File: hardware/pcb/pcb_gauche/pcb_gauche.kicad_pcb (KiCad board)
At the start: 2 copper layers, 28 x 56 mm, 14 parts, among them P1 TE-FFC-10-0.5

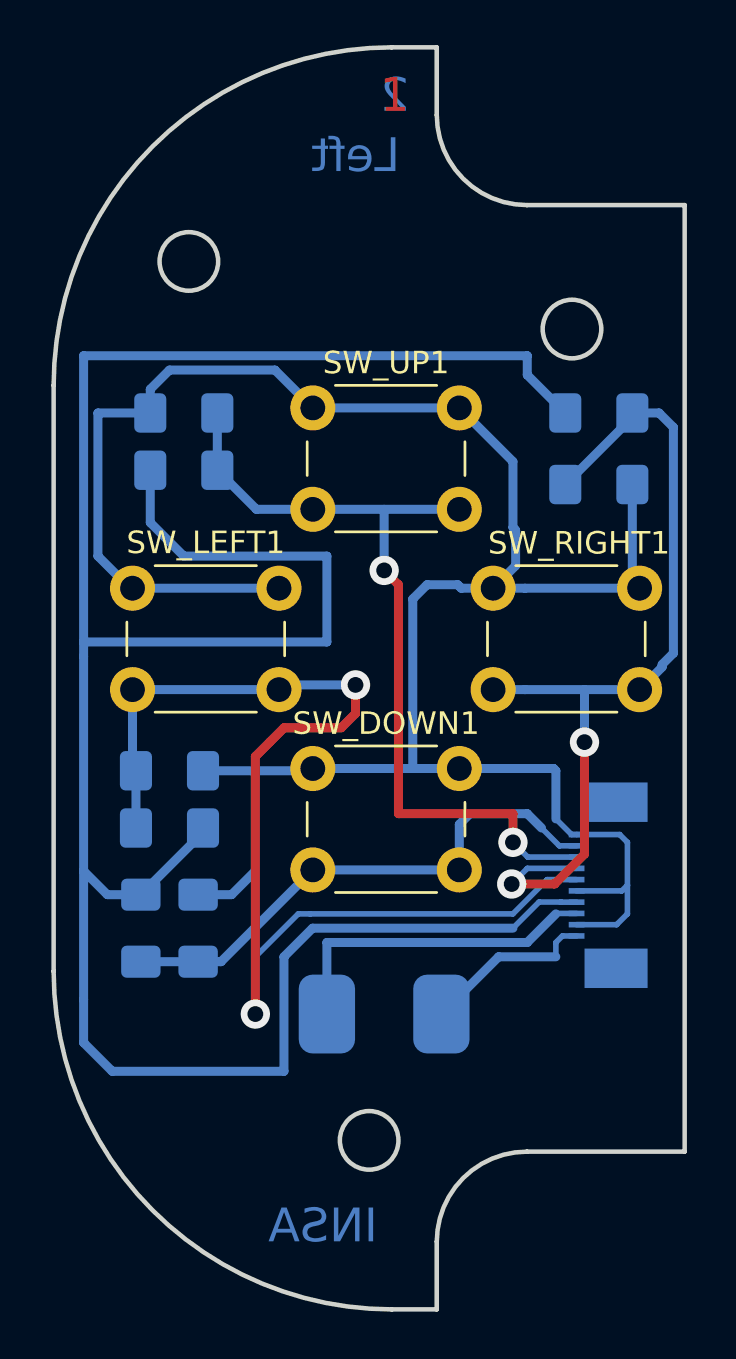
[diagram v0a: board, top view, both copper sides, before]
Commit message: mise a jour des pcb et design mecaniques
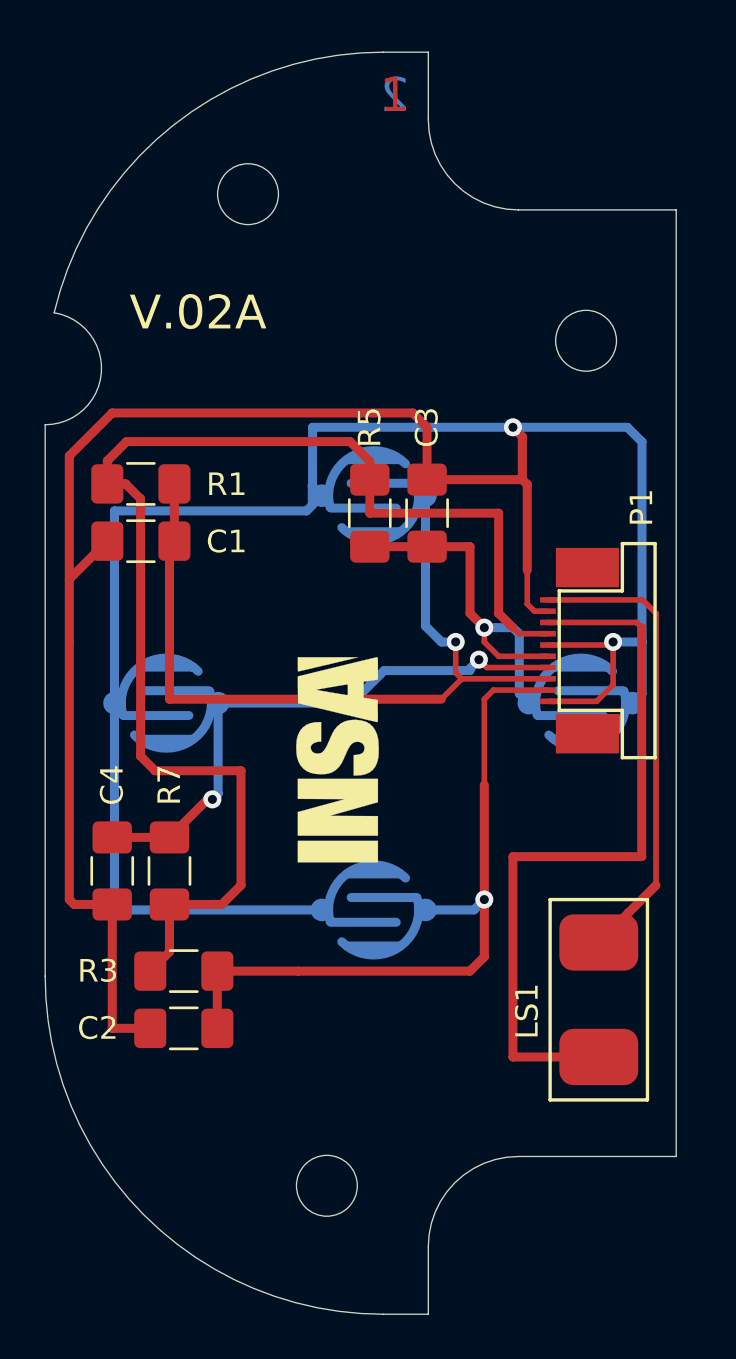
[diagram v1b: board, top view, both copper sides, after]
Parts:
- added Logo1: LOGO, Insa:insa-image, F.Cu at (129.8, 104.5)
- added REF**: MountingHole_2.7mm_M2.5, MountingHole:MountingHole_2.7mm_M2.5, F.Cu at (140.6, 86.0)
- added REF**: MountingHole_2.7mm_M2.5, MountingHole:MountingHole_2.7mm_M2.5, F.Cu at (125.6, 79.5)
- added REF**: MountingHole_2.7mm_M2.5, MountingHole:MountingHole_2.7mm_M2.5, F.Cu at (129.1, 123.5)
- C1, C2, C3, C4, LS1, P1, R1, R3, R5, R7: moved to F.Cu
- SW_DOWN1, SW_LEFT1, SW_RIGHT1, SW_UP1: footprint Button_Switch_THT:SW_PUSH_6mm -> Insa:RubberKey-4mm-2; moved to B.Cu
- moved R7 27.9 mm to (122.1, 109.5), turned to 90 degrees
- moved C4 27.6 mm to (119.6, 109.5), turned to 270 degrees
- moved SW_LEFT1 20.5 mm to (140.4, 102.1)
- moved R5 16.6 mm to (131.0, 93.7), turned to 270 degrees
- moved C3 16.2 mm to (133.6, 93.7), turned to 90 degrees
- moved SW_RIGHT1 15.4 mm to (122.0, 102.1), turned to 180 degrees
- moved P1 10.5 mm to (139.3, 99.8), turned to 270 degrees
- moved LS1 9.55 mm to (141.2, 115.3), turned to 270 degrees
- moved SW_DOWN1 6.83 mm to (131.2, 111.3), turned to 180 degrees
- moved C1 6.00 mm to (120.9, 94.9)
- moved SW_UP1 4.74 mm to (131.2, 92.9), turned to 180 degrees
- moved C2 4.49 mm to (122.8, 116.5), turned to 180 degrees
- moved R3 2.69 mm to (122.8, 114.0), turned to 0 degrees
- moved R1 2.00 mm to (120.9, 92.4)
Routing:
- net VCC: track 114.4 -> 58.2 mm
- net GND: track 102.1 -> 139.5 mm, vias 0 -> 2
- net /Key_Left: track 52.3 -> 16.9 mm, vias 2 -> 1
- net /Audio_Left_2: track 14.8 -> 32.8 mm
- net /Key_Right: track 39.5 -> 25.2 mm
- net /Audio_Left_1: track 7.81 -> 20.7 mm
- net /Key_Down: track 23.8 -> 31.9 mm, vias 0 -> 1
- net /Key_Up: track 37.2 -> 35.2 mm, vias 2 -> 1
- net (no net): track 0.00 -> 1.13 mm
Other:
- outline, holes or cut-outs redrawn
- board text added: "V.02A"
- board text removed: "INSA"
- board text removed: "Left"
